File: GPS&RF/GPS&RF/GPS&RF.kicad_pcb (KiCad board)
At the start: 2 copper layers, 52.8 x 49.5 mm, 13 parts, among them IC1 FGPMMOPA6H, J1 U.FL-R-SMT(10), J2 Conn_01x13_Male, U1 LAMBDA-9S-Global

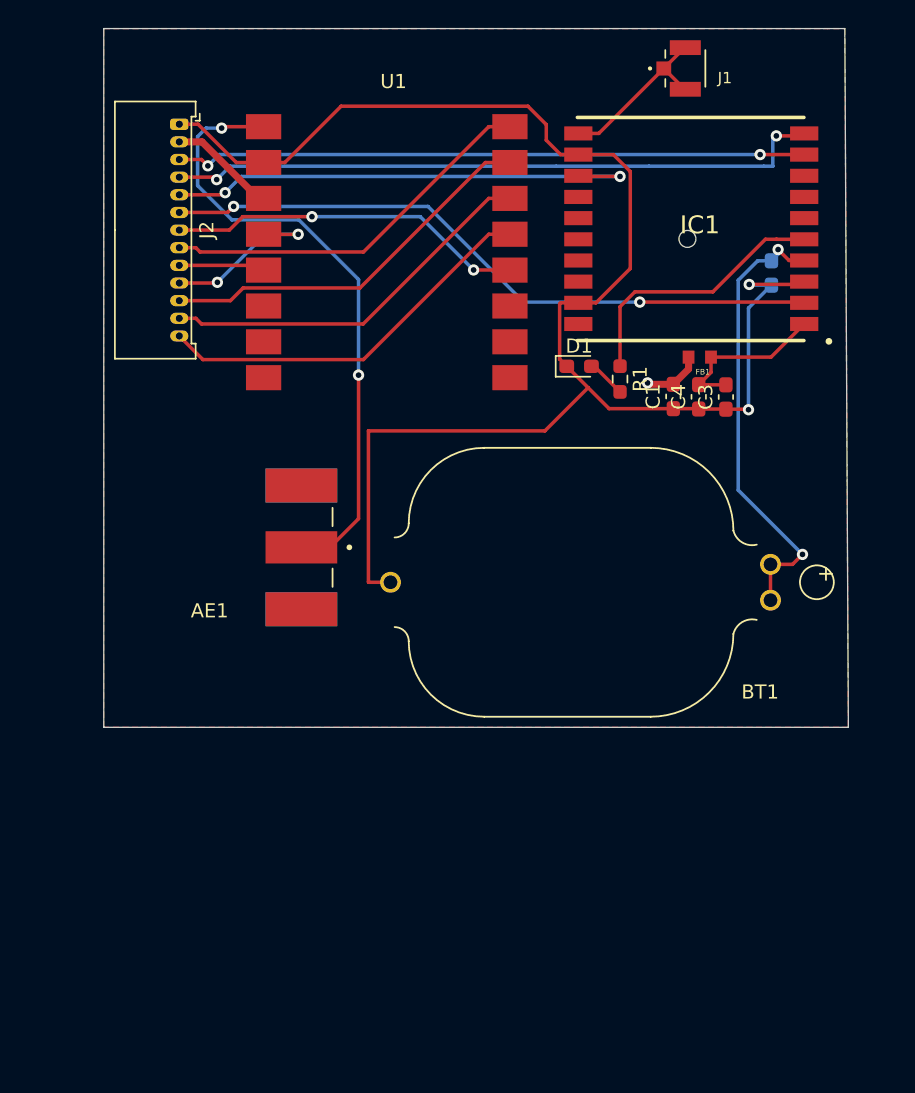
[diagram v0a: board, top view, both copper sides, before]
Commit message: COMPLETED RF&GPS BOARD!
hoooorahhhh
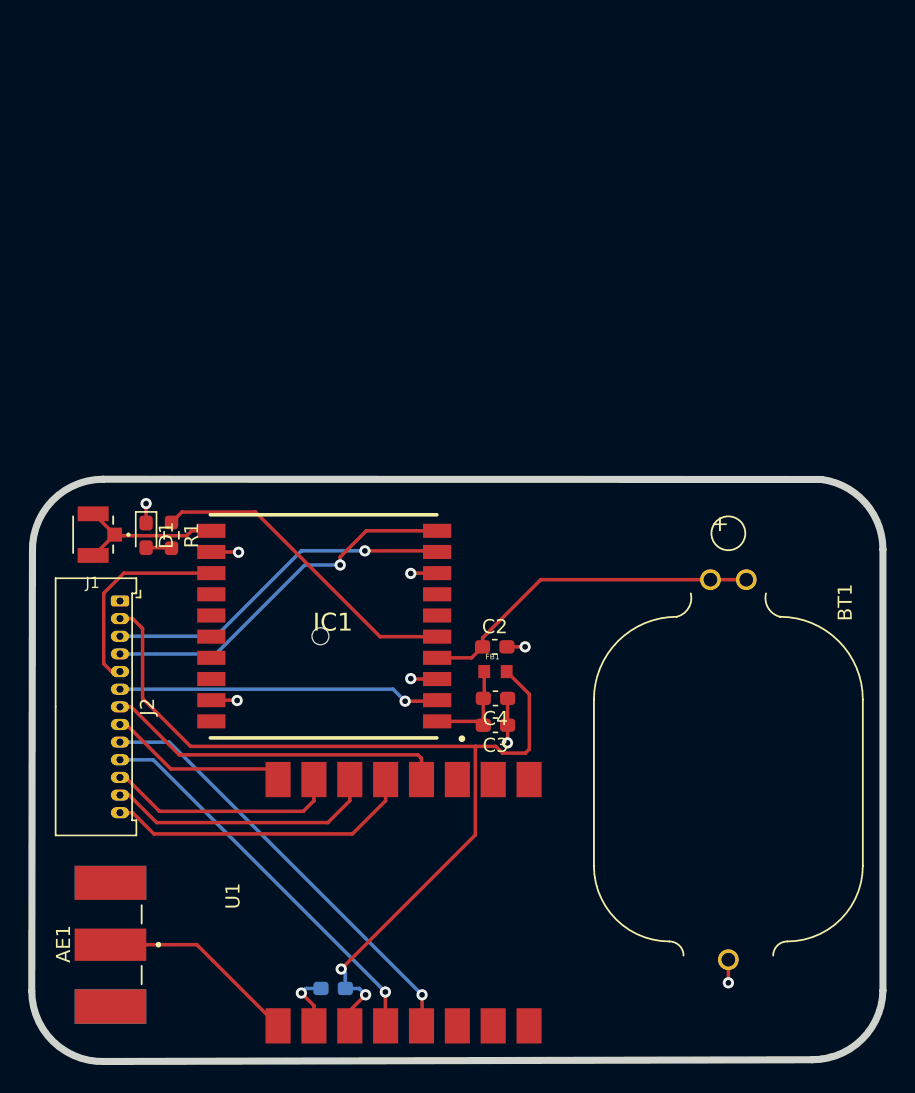
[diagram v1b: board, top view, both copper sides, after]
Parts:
- C1: moved to B.Cu
- C2: moved to F.Cu
- moved U1 63.7 mm to (144.6, 133.4), turned to 90 degrees
- moved J1 53.4 mm to (131.5, 98.6), turned to 180 degrees
- moved C1 48.4 mm to (148.5, 130.8), turned to 0 degrees
- moved IC1 38.3 mm to (139.8, 113.0)
- moved J2 34.0 mm to (133.4, 103.3)
- moved R1 33.6 mm to (137.1, 98.7)
- moved C2 33.0 mm to (159.9, 106.5), turned to 0 degrees
- moved D1 32.9 mm to (135.2, 98.7), turned to 270 degrees
- moved AE1 31.2 mm to (132.7, 127.7)
- moved C3 28.4 mm to (160.0, 112.1), turned to 180 degrees
- moved FB1 26.6 mm to (160.0, 108.3), turned to 0 degrees
- moved C4 25.8 mm to (160.0, 110.2), turned to 180 degrees
- moved BT1 16.9 mm to (176.5, 115.2), turned to 270 degrees
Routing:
- net GND: track 113.2 -> 19.2 mm, vias 2 -> 9
- net +3V3: track 11.9 -> 67.6 mm, vias 1 -> 2
- net Net-(AE1-Pad1): track 44.4 -> 14.3 mm, vias 2 -> 0
- net /RX_D1: track 6.11 -> 31.0 mm, vias 0 -> 1
- net /GPSRST: track 47.3 -> 22.9 mm, vias 2 -> 1
- net /TX_D2: track 46.8 -> 26.4 mm, vias 2 -> 1
- net /1PPS: track 34.7 -> 14.6 mm, vias 2 -> 0
- net /RX_D2: track 44.8 -> 25.3 mm, vias 2 -> 1
- net /TX_D1: track 12.3 -> 28.0 mm, vias 2 -> 1
- net /CS: track 27.2 -> 12.8 mm
- net /MOSI: track 27.5 -> 16.5 mm
- net /MISO: track 27.3 -> 19.2 mm
- net Net-(BT1-Pad+1): track 32.5 -> 24.6 mm, vias 2 -> 0
- net /SCK: track 27.8 -> 21.9 mm
- net Net-(C3-Pad2): track 11.8 -> 7.21 mm
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- added copper zone on B.Cu, net GND
- added copper zone on F.Cu, net GND
- removed copper zone on F.Cu, net +3V3
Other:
- board size 52.8 x 49.5 mm -> 60.3 x 41.2 mm
- board text added: "HOLA"
- board text added: "RF & GPS"
